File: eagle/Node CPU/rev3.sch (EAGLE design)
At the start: 44 parts, among them IC1 MEGA8-AI

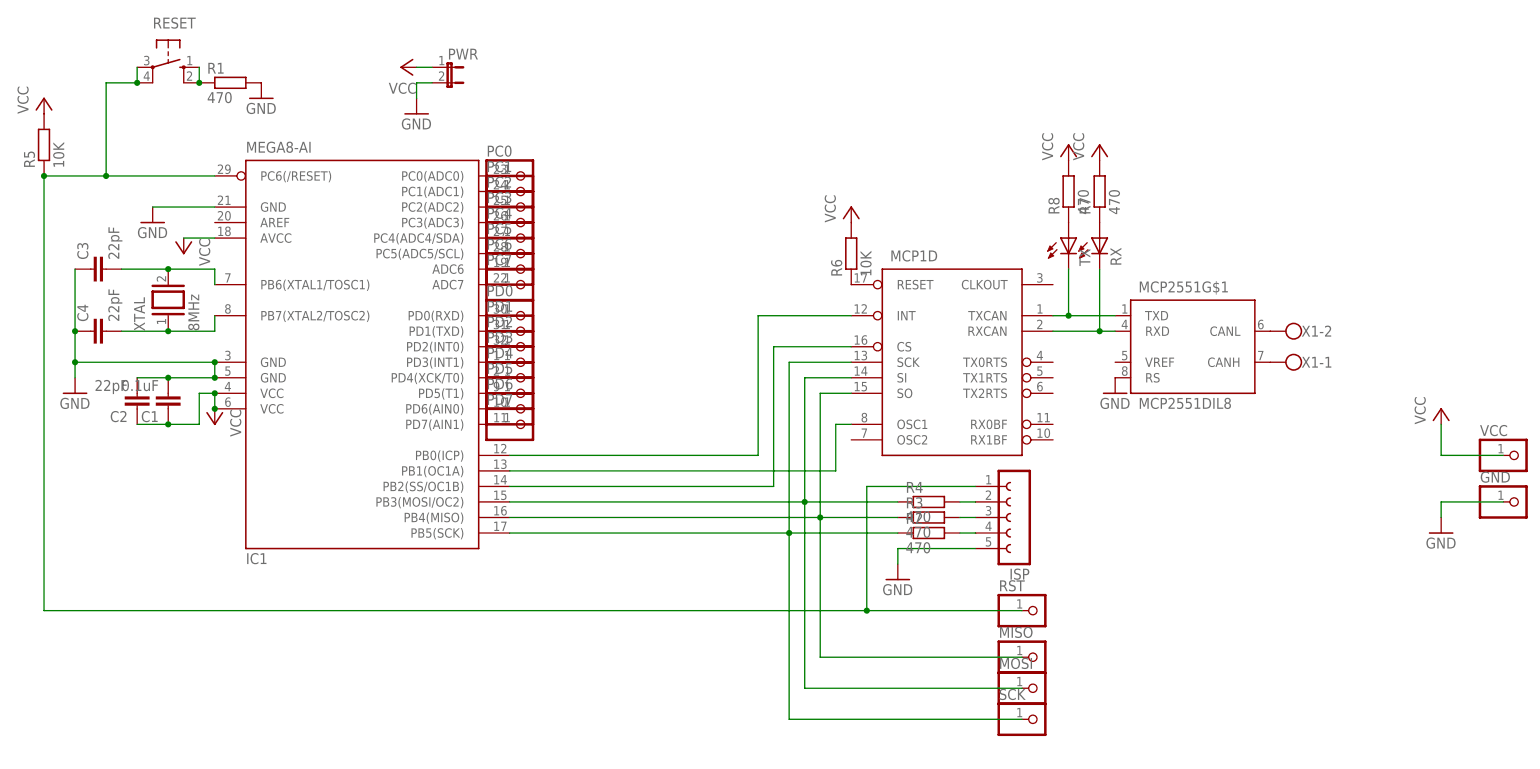
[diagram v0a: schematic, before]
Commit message: updated to revision 3 of the board
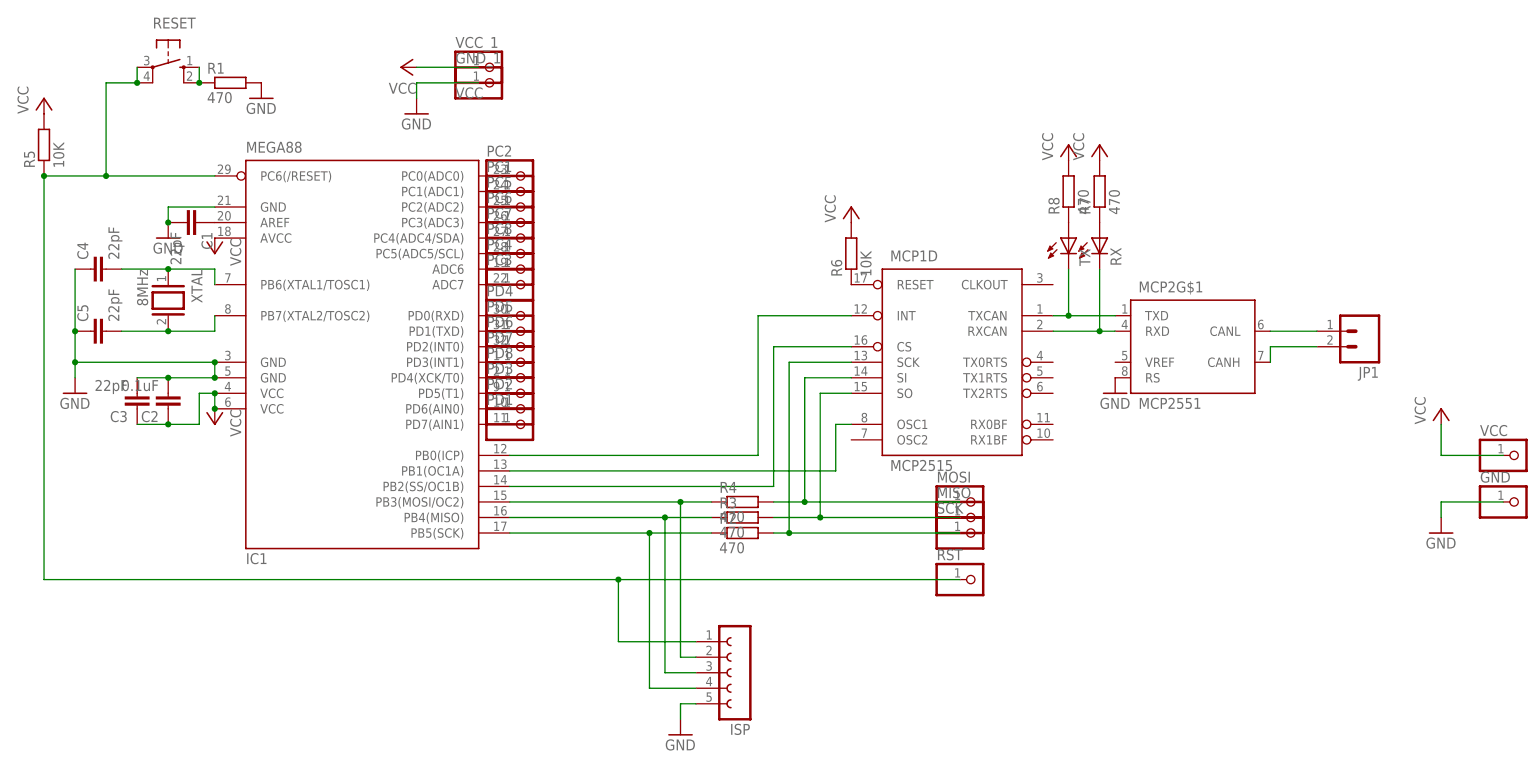
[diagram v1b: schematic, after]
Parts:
- removed PC0, PD0: (no value), pinhead:PINHD-1X1
- removed PWR: (no value), SparkFun-Passives:JUMPER-2PTH
- removed X1: (no value), con-wago-500:W237-102
- added C5: 22pF, resistor:C-EUC0603
- added GND_1, PC8, PD8: (no value), pinhead:PINHD-1X1
- added JP1: (no value), SparkFun-Connectors:M023.5MM
- added VCC_1: VCC, pinhead:PINHD-1X1
- C1: value 0.1uF -> 22pF
- C2: value 22pF -> 0.1uF
- IC1: value MEGA8-AI -> MEGA88
- MCP1: value (none) -> MCP2515
- MCP2: value MCP2551DIL8 -> MCP2551
- renumbered MCP2551 to MCP2
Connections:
- removed net N$36: MCP2G$1.CANL, X1-2.KL
- new net N$38: MCP1D.SO, MISO.1, R3.2
- new net N$39: IC1.PB5(SCK), ISP.4, R2.1
- net GND: now also C3.2, C5.1, GND_1.1; no longer C3.1, PWR.2
- net N$1: now also C1.1, IC1.AREF; no longer IC1.PB5(SCK), MCP1D.SCK, R2.1, SCK.1
- net N$10: now also JP1.1, MCP2G$1.CANL; no longer C3.2, IC1.PB6(XTAL1/TOSC1), XTAL.2
- net N$15: now also MCP1D.SCK, R2.2, SCK.1; no longer ISP.2, R4.2
- net N$16: now also JP1.2, MCP2G$1.CANH; no longer ISP.3, R3.2
- net N$17: now also IC1.PB3(MOSI/OC2), ISP.2, R4.1; no longer ISP.4, R2.2
- net N$2: now also ISP.3; no longer MCP1D.SO, MISO.1
- net N$20: now also PC2.1; no longer PC0.1
- net N$22: now also PC5.1; no longer PC2.1
- net N$23: now also PC6.1; no longer PC3.1
- net N$24: now also PC7.1; no longer PC4.1
- net N$25: now also PC8.1; no longer PC5.1
- net N$26: now also PC4.1; no longer PC6.1
- net N$27: now also PC3.1; no longer PC7.1
- net N$28: now also PD4.1; no longer PD0.1
- net N$29: now also PD5.1; no longer PD1.1
- net N$3: now also R4.2; no longer IC1.PB3(MOSI/OC2), R4.1
- net N$30: now also PD6.1; no longer PD2.1
- net N$31: now also PD7.1; no longer PD3.1
- net N$32: now also PD8.1; no longer PD4.1
- net N$33: now also PD3.1; no longer PD5.1
- net N$34: now also PD2.1; no longer PD6.1
- net N$35: now also PD1.1; no longer PD7.1
- net N$37: now also C4.2, IC1.PB6(XTAL1/TOSC1), XTAL.1; no longer MCP2G$1.CANH, X1-1.KL
- net N$9: now also C5.2, XTAL.2; no longer C4.2, XTAL.1
- net VCC: now also C3.1, VCC_1.1; no longer C1.1, PWR.1
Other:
- moved on the sheet: C1, C2, C3, C4, ISP, MISO, MOSI, PC2, PC3, PC4, PC5, PC6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
